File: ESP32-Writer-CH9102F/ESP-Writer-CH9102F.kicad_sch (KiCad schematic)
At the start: 31 parts, among them J1 USB2.0-C_SMT, J2 ESP-Prog-ProgramCOM_SEND, SW1 SW_Push, U1 CH9102F, U2 CH32V003J4M6, U3 CH213K, U4 AMS1117

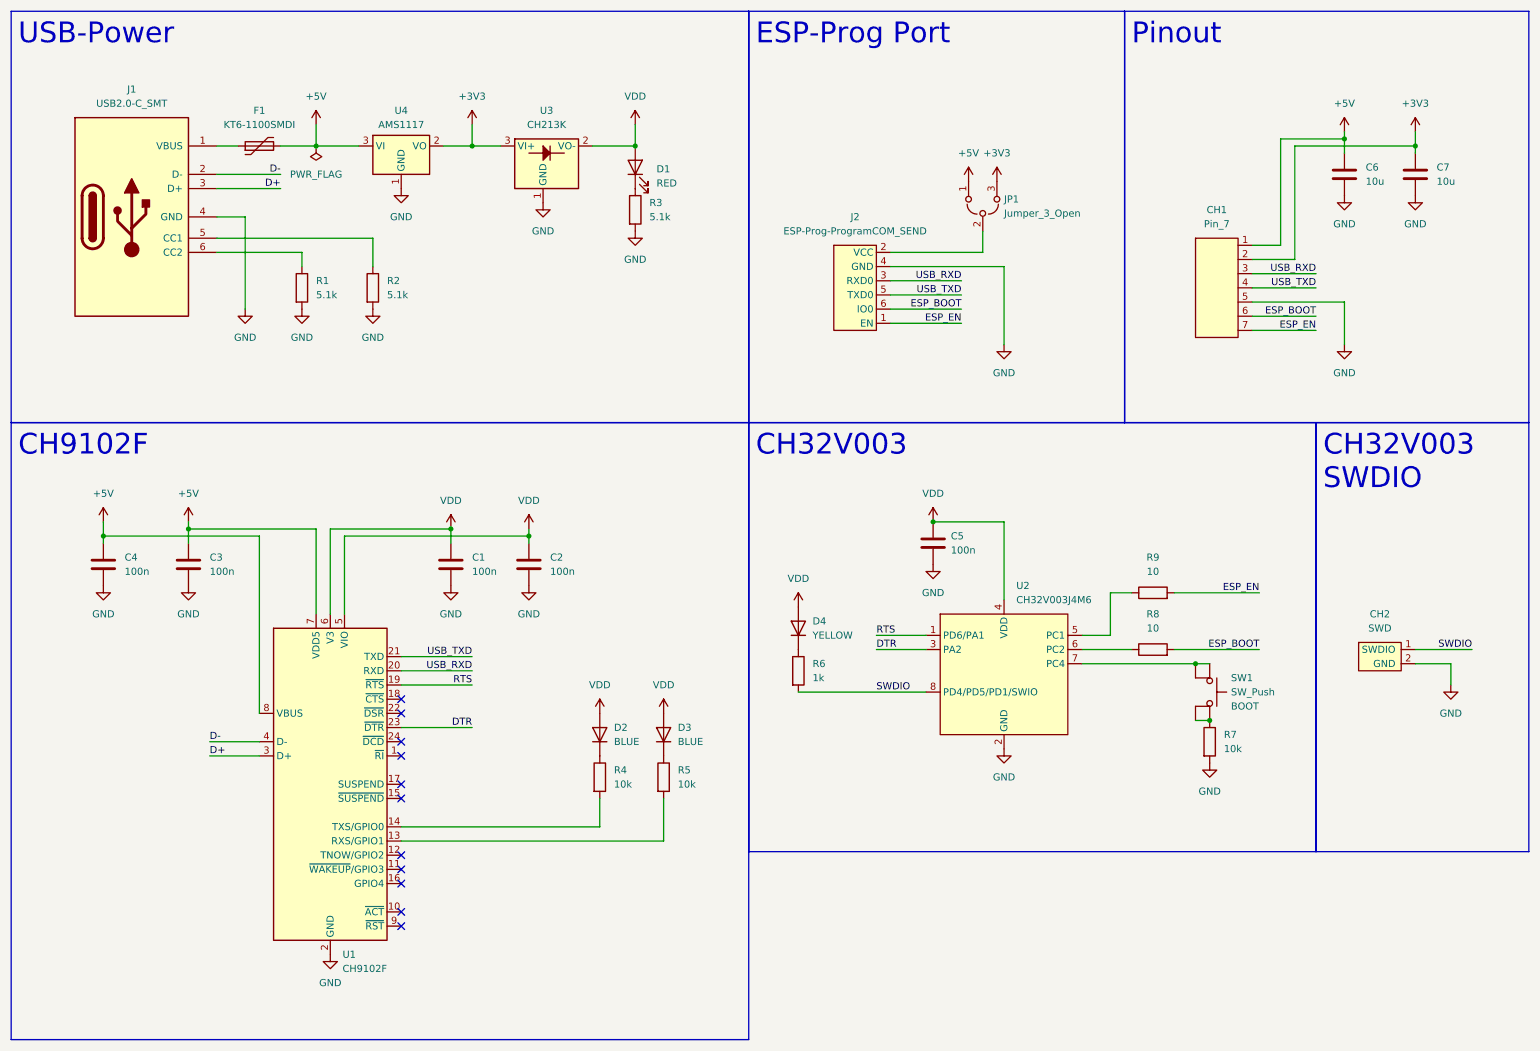
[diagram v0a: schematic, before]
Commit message: esp32-writer-ch9102f/v1.1.0
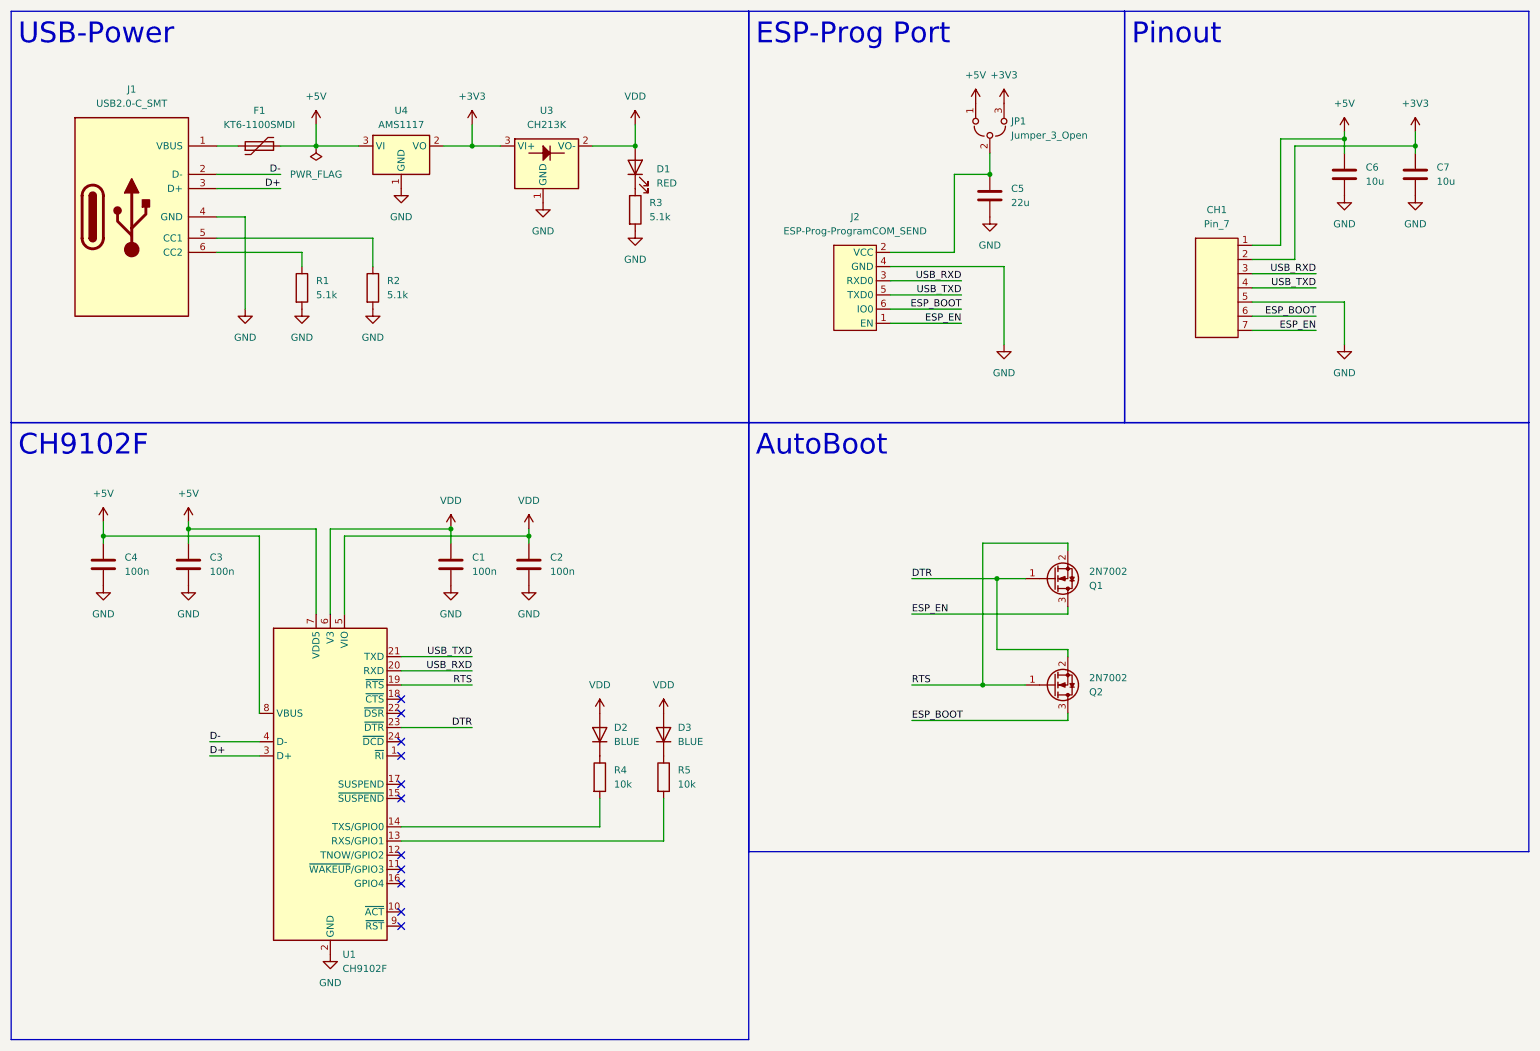
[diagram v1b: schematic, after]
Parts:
- removed CH2: SWD, 74th:PinOut_Pin_2, symbol 74th_Interface:SWD_WCH-1Wire
- removed D4: YELLOW, 74th:LED_0805_2012, symbol Device:D
- removed R6: 1k, 74th:Register_0603_1608, symbol Device:R
- removed R7: 10k, 74th:Register_0603_1608, symbol Device:R
- removed R8, R9: 10, 74th:Register_0603_1608, symbol Device:R
- removed SW1: SW_Push, 74th:Switch_SKRPABE010_Pin-4, symbol 74th_Interface:SW_Push_Pin-4
- removed U2: CH32V003J4M6, 74th:Package_SOIC-8_3.9x4.9mm_P1.27mm, symbol 74th_MCU:CH32V003J4M6
- added Q1, Q2: 2N7002, 74th:Package_SOT-23, symbol Transistor_FET:2N7002
- C5: value 100n -> 22u
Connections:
- net DTR: now also Q1.1 (G), Q2.2 (S)
- net ESP_BOOT: now also Q2.3 (D)
- net ESP_EN: now also Q1.3 (D)
- net RTS: now also Q1.2 (S), Q2.1 (G)
- net VDD: no longer C5.1
- net at J2.2 (VCC), JP1.2 (C): now also C5.1
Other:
- note added: "AutoBoot"
- note removed: "CH32V003"
- note removed: "CH32V003 SWDIO"
- moved on the sheet: JP1
